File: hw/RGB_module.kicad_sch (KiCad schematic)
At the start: 10 parts, among them J1 Conn_01x04, J2 Conn_01x04, U1 ZSCS-2016C-08D-Z4

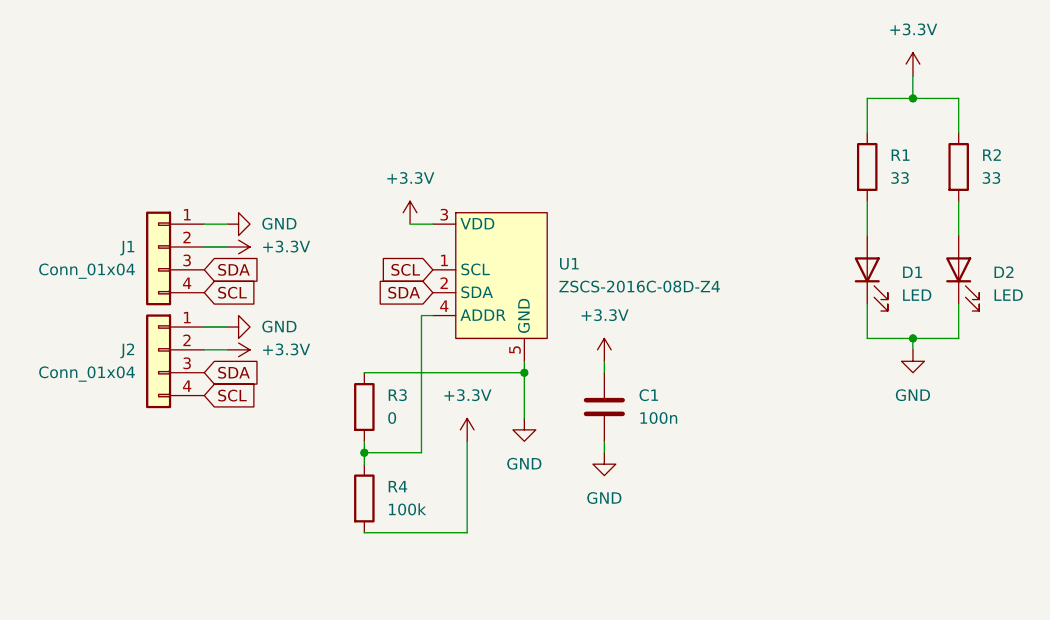
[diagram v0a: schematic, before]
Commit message: board_v3
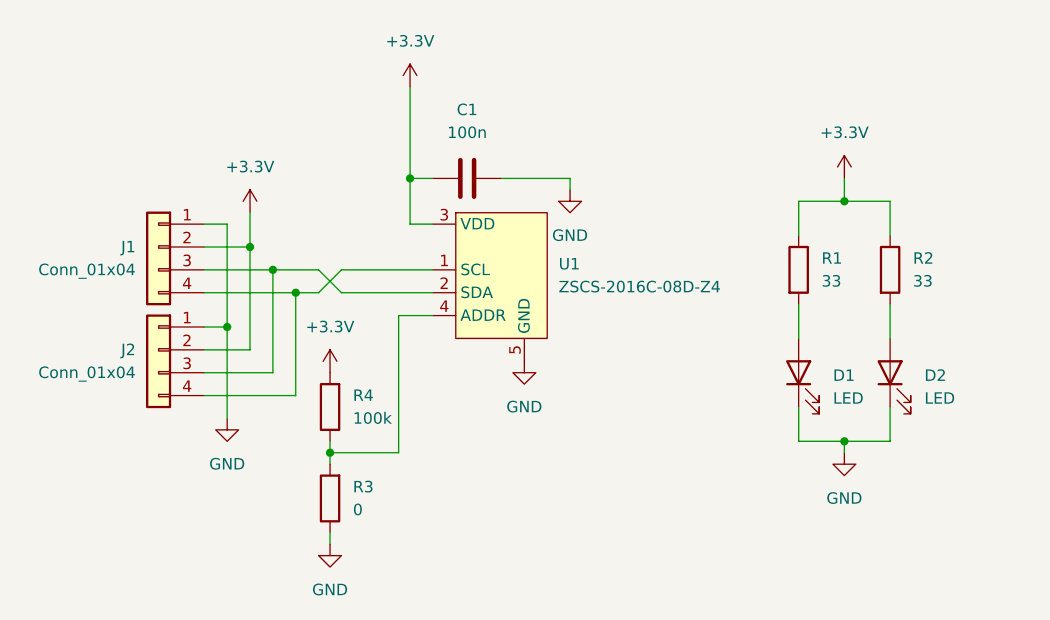
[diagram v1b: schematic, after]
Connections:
- net SCL: no longer names the net of J1.4 (Pin_4), J2.4 (Pin_4), U1.1 (SCL)
- net SDA: no longer names the net of J1.3 (Pin_3), J2.3 (Pin_3), U1.2 (SDA)
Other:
- moved on the sheet: C1, D1, D2, R1, R2, R3, R4
